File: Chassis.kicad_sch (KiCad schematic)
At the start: 15 parts, among them J1 Conn_01x02, J10 Conn_01x02, J2 Conn_01x02, J3 Conn_01x02, J4 Conn_01x02, J5 Conn_01x02, J6 Conn_01x02, J7 Conn_01x02, J8 Conn_01x02, J9 Conn_01x02

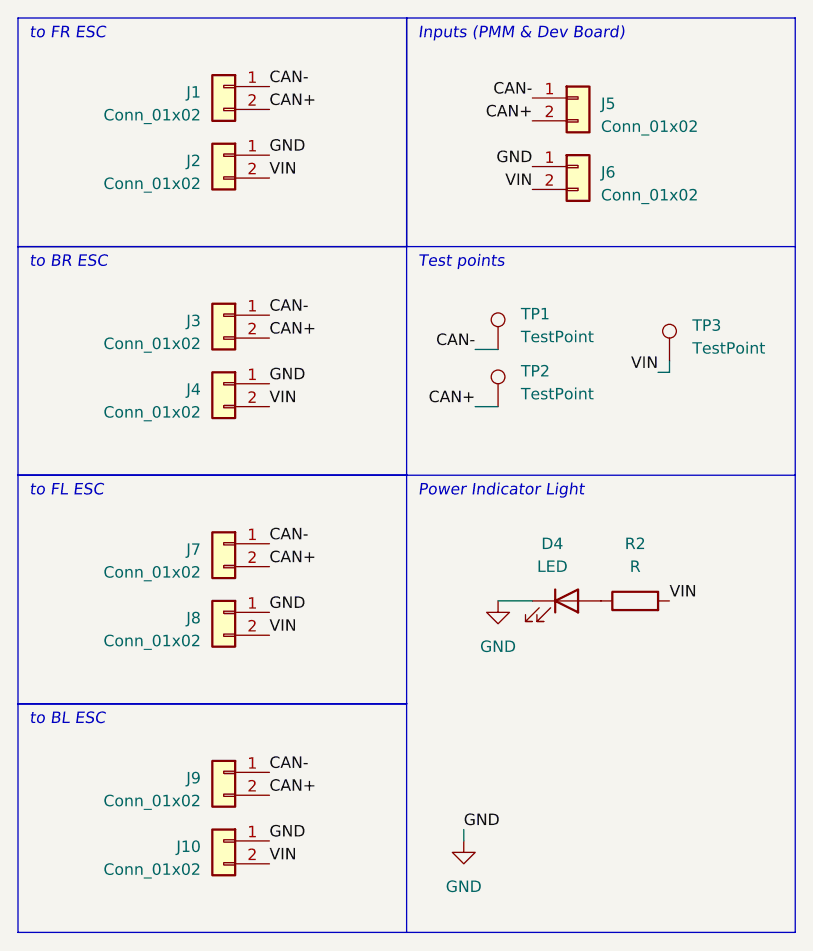
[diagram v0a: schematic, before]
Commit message: Completed initial layout
I'm going to get roasted over some of these choices
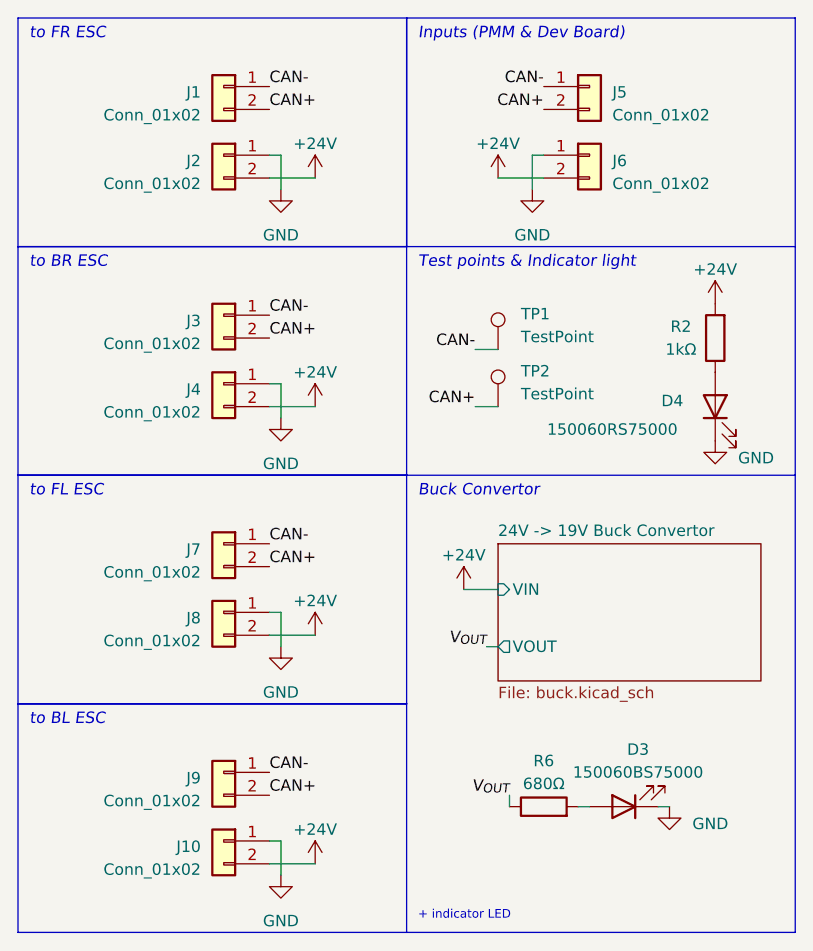
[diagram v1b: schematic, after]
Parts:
- removed TP3: TestPoint, TestPoint:TestPoint_Pad_1.0x1.0mm, symbol Connector:TestPoint
- added D3: 150060BS75000, LED_SMD:LED_0603_1608Metric_Pad1.05x0.95mm_HandSolder, symbol Device:LED
- added R6: 680Ω, Resistor_SMD:R_0603_1608Metric_Pad0.98x0.95mm_HandSolder, symbol Device:R
- D4: value LED -> 150060RS75000
- R2: value R -> 1kΩ
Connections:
- net GND: now also D3.1 (K)
- net VIN renamed +24V
- new net: D3.2 (A), R6.2
- new net V_{OUT}: R6.1
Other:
- added sheet 24V -> 19V Buck Convertor (buck.kicad_sch)
- note added: "+ indicator LED"
- note added: "Buck Convertor"
- note added: "Test points & Indicator light"
- note removed: "Power Indicator Light"
- note removed: "Test points"
- moved on the sheet: D4, J5, J6, R2
